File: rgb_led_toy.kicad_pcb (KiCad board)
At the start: 2 copper layers, 43.4 x 43.4 mm, 72 parts, among them IC1 AT168, IC2 MBI5168, IC3 MBI5168, IC4 MBI5168, P1 I2C, P2 PORTC, P3 FTDI, U1 MADW__TSOP38238

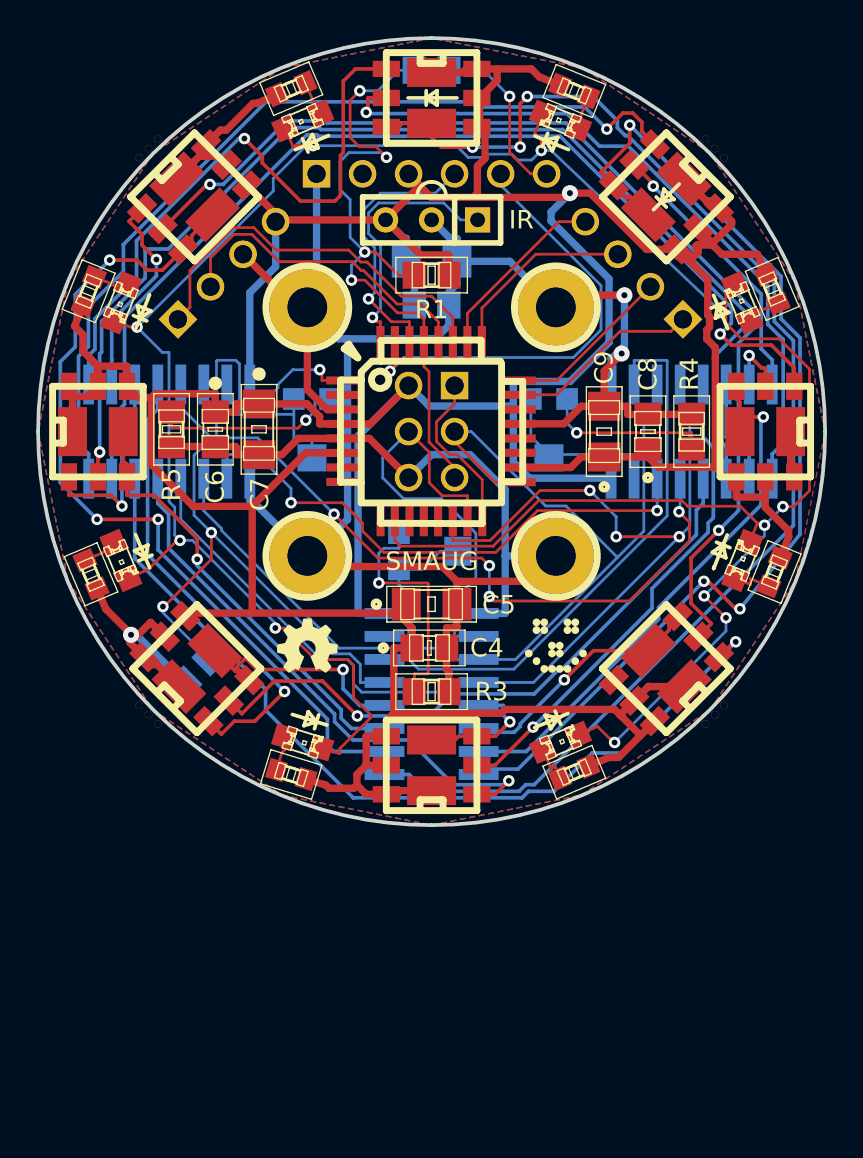
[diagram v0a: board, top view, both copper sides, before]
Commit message: V3.0 doodles.
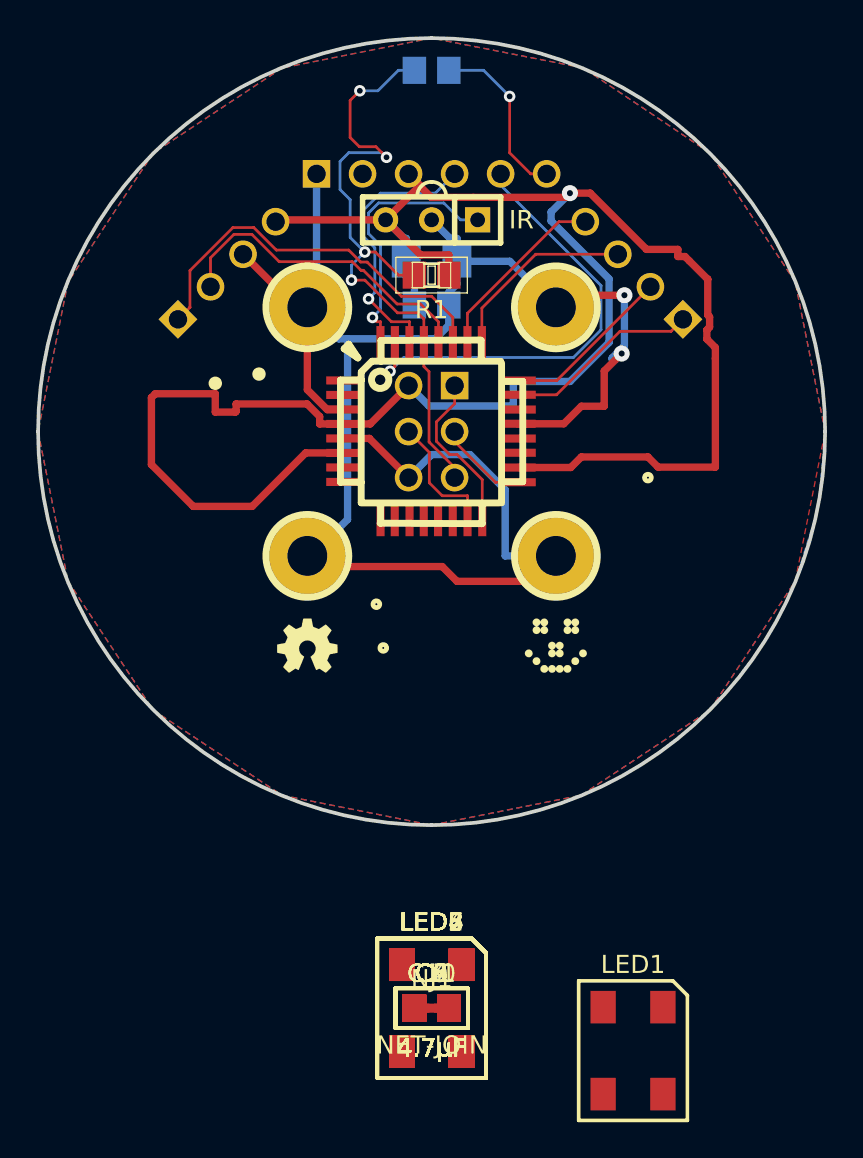
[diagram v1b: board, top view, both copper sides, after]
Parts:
- removed D1, D2, D3, D4, D5, D6, D7, D8: RGB_SMD, MADW__PLCC6-5050_PLCC2_DUAL
- removed D10, D11, D12, D13, D14, D15, D16, D9: LED, -CHIPLED_0805
- removed DRL1, DRL10, DRL11, DRL12, DRL2, DRL3, DRL4, DRL5, DRL6, DRL7, DRL8, DRL9: 1PIN, 1pin
- removed G3, G4, G5, G6: LOGO, LOGO
- removed IC2, IC3, IC4: MBI5168, MADW__SO16
- removed R10, R11, R12, R13, R6, R7, R8, R9: R, -R0603
- removed R2: 10k, -R0805
- removed R3, R4, R5: 600R, -R0805
- removed RV1, RV2, RV3: 4k7, MADW__TC33X-POT
- added C10, C11: 4.7µF, MADW__C0805, F.Cu at (83.2, 102.6)
- added LED1: MADW__WS2812B, MADW__PLCC4-5050, F.Cu at (94.3, 104.9)
- added LED2, LED3, LED4, LED5, LED6, LED7, LED8: MADW__WS2812B, MADW__PLCC4-5050, F.Cu at (83.2, 102.6)
- added NJ1: NET-JOIN, MADW__SMD-net-noin-0.5mm, F.Cu at (83.2, 102.6)
- C4, C6, C8: value 100nF -> 4.7µF; footprint -C0805 -> MADW__C0805
- C5, C7, C9: value 10µF -> 4.7µF; footprint -C1206 -> MADW__C0805
- moved C6 34.1 mm to (83.2, 102.6), turned to 0 degrees
- moved C8 34.0 mm to (83.2, 102.6), turned to 0 degrees
- moved C7 33.3 mm to (83.2, 102.6), turned to 0 degrees
- moved C9 33.2 mm to (83.2, 102.6), turned to 0 degrees
- moved C5 22.3 mm to (83.2, 102.6)
- moved C4 19.9 mm to (83.2, 102.6)
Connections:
- C4 pad 2: GND -> GNDPWR
- C5 pad 2: GND -> GNDPWR
- C6 pad 2: GND -> GNDPWR
- C7 pad 2: GND -> GNDPWR
- C8 pad 2: GND -> GNDPWR
- C9 pad 2: GND -> GNDPWR
- IC1 pad 1: /OE -> (no net)
- IC1 pad 10: /led0 -> (no net)
- IC1 pad 12: (no net) -> /DATA
- IC1 pad 14: /LATCH -> (no net)
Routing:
- net VCC: track 300.5 -> 118.8 mm, vias 2 -> 1
- net /led0: track 144.9 -> 0.00 mm, vias 11 -> 0
- net /OE: track 84.0 -> 0.00 mm, vias 7 -> 0
- net /O1.4: track 72.4 -> 0.00 mm, vias 3 -> 0
- net /O2.6: track 63.8 -> 0.00 mm, vias 1 -> 0
- net /LATCH: track 63.3 -> 0.00 mm, vias 3 -> 0
- net /O3.2: track 58.4 -> 0.00 mm, vias 1 -> 0
- net /O1.3: track 58.3 -> 0.00 mm, vias 3 -> 0
- net /SCK: track 57.7 -> 4.96 mm
- net /O2.5: track 49.3 -> 0.00 mm, vias 1 -> 0
- net /O3.3: track 48.8 -> 0.00 mm, vias 1 -> 0
- net /O3.1: track 48.6 -> 0.00 mm, vias 1 -> 0
- net /O1.5: track 46.6 -> 0.00 mm, vias 3 -> 0
- net /O2.4: track 39.2 -> 0.00 mm, vias 1 -> 0
- net /O2.7: track 35.0 -> 0.00 mm, vias 1 -> 0
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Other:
- board text removed: "ADJ."
- board text removed: "Dori"
- board text removed: "ISP"
- board text removed: "Nori"
- board text removed: "Ori"
- board text removed: "PLCC2"
- board text removed: "SMAUG"

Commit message: Might be a first working V3.0
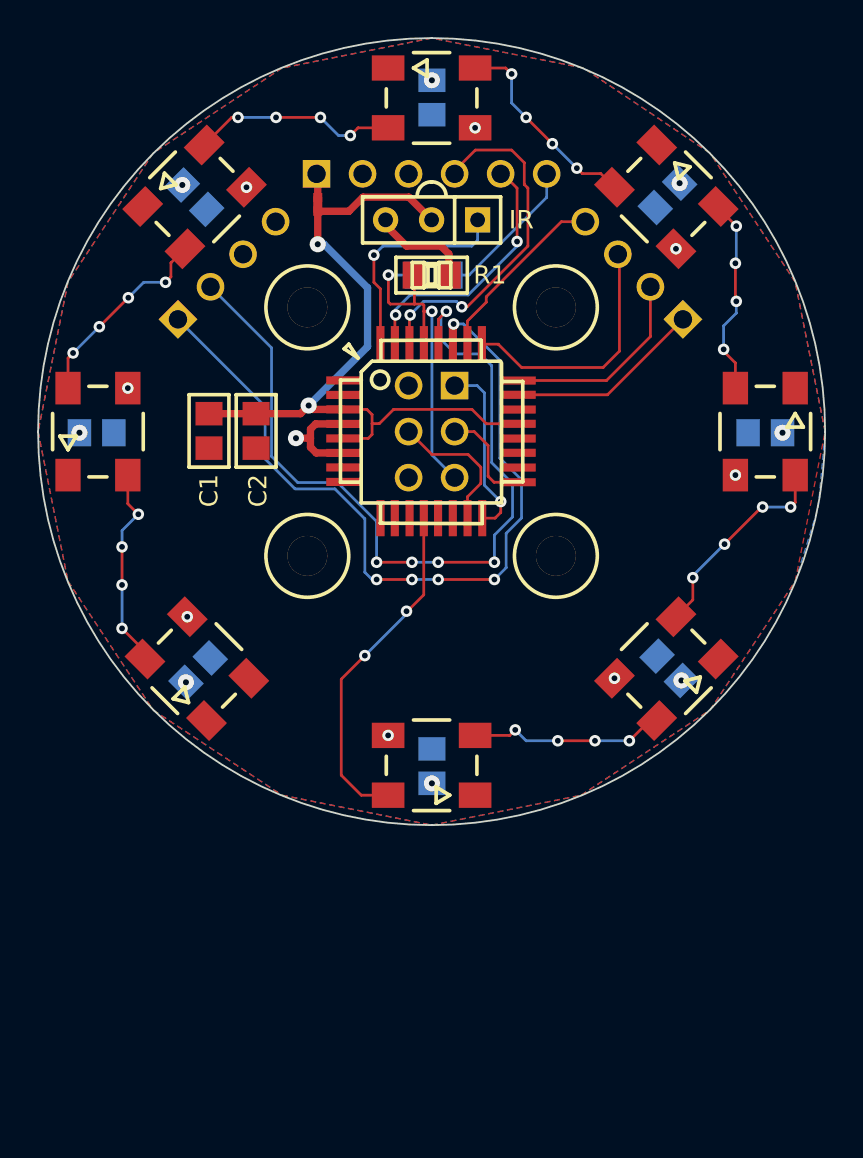
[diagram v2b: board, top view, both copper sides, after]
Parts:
- removed G1: LOGO, LOGO
- removed G2: LOGO, 
- C1: footprint -C0805 -> MADW__C0805; moved to F.Cu
- C10, C11, C4, C5, C6, C7, C8, C9: moved to B.Cu
- C2: footprint -C1206 -> MADW__C0805; moved to F.Cu
- C3: footprint -C0805 -> MADW__C0805
- R1: footprint -R0805 -> MADW__R0805
- moved C8 50.3 mm to (83.2, 52.3), turned to 270 degrees
- moved LED5 50.2 mm to (83.2, 52.3), turned to 90 degrees
- moved C7 46.7 mm to (96.2, 57.7), turned to 225 degrees
- moved LED6 46.6 mm to (70.1, 57.8), turned to 135 degrees
- moved C9 46.6 mm to (70.1, 57.8), turned to 315 degrees
- moved LED4 46.6 mm to (96.1, 57.8), turned to 45 degrees
- moved NJ1 44.8 mm to (76.9, 58.2), turned to 90 degrees
- moved LED3 36.8 mm to (101.6, 70.7)
- moved LED7 36.8 mm to (64.8, 70.7), turned to 180 degrees
- moved C10 36.7 mm to (64.7, 70.8)
- moved C6 36.7 mm to (101.6, 70.8), turned to 180 degrees
- moved C5 22.9 mm to (96.3, 83.8), turned to 135 degrees
- moved LED8 22.8 mm to (70.2, 83.8), turned to 225 degrees
- moved LED2 22.8 mm to (96.1, 83.8), turned to 315 degrees
- moved C11 22.7 mm to (70.3, 83.9), turned to 45 degrees
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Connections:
- JP1 pad 6: GND -> GNDPWR
- P1 pad 3: GND -> GNDPWR
- P3 pad 1: GND -> GNDPWR
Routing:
- net VCC: track 118.8 -> 11.8 mm, vias 1 -> 9
- net GND: track 104.0 -> 41.5 mm
- net /SCL: track 17.9 -> 45.7 mm, vias 0 -> 5
- net /SDA: track 22.0 -> 44.9 mm, vias 0 -> 5
- net /DATA: track 0.00 -> 19.1 mm, vias 0 -> 2
- net /RESET: track 36.6 -> 19.0 mm, vias 4 -> 2
- net N-000007: track 0.00 -> 11.7 mm, vias 0 -> 4
- net N-000009: track 0.00 -> 11.4 mm, vias 0 -> 4
- net N-000003: track 0.00 -> 11.4 mm, vias 0 -> 4
- net N-000001: track 0.00 -> 11.3 mm, vias 0 -> 4
- net N-000008: track 0.00 -> 11.1 mm, vias 0 -> 4
- net N-000005: track 0.00 -> 11.0 mm, vias 0 -> 4
- net N-000006: track 0.00 -> 10.9 mm, vias 0 -> 4
- net /TXO: track 25.1 -> 14.5 mm, vias 1 -> 2
- net /RXI: track 15.2 -> 19.4 mm, vias 1 -> 2
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- added copper zone on B.Cu, net GNDPWR
- added copper zone on F.Cu, net VCC
- removed copper zone on B.Cu, net (none)
- removed copper zone on F.Cu, net (none)
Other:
- board text added: "2013 V3.0.a"
- board text added: "blog.spitzenpfeil.org"
- board text removed: "2012 V2.1"
- board text removed: "blog. spitzenpfeil .org"
